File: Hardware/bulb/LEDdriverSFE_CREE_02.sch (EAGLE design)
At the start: 27 parts, among them U1 ZXLD1360, U2 ZXLD1360, U3 ZXLD1360, U4 ZXLD1360, U5 SFW10R-1STE1LF, X1 52745-1090, X2 52745-1090

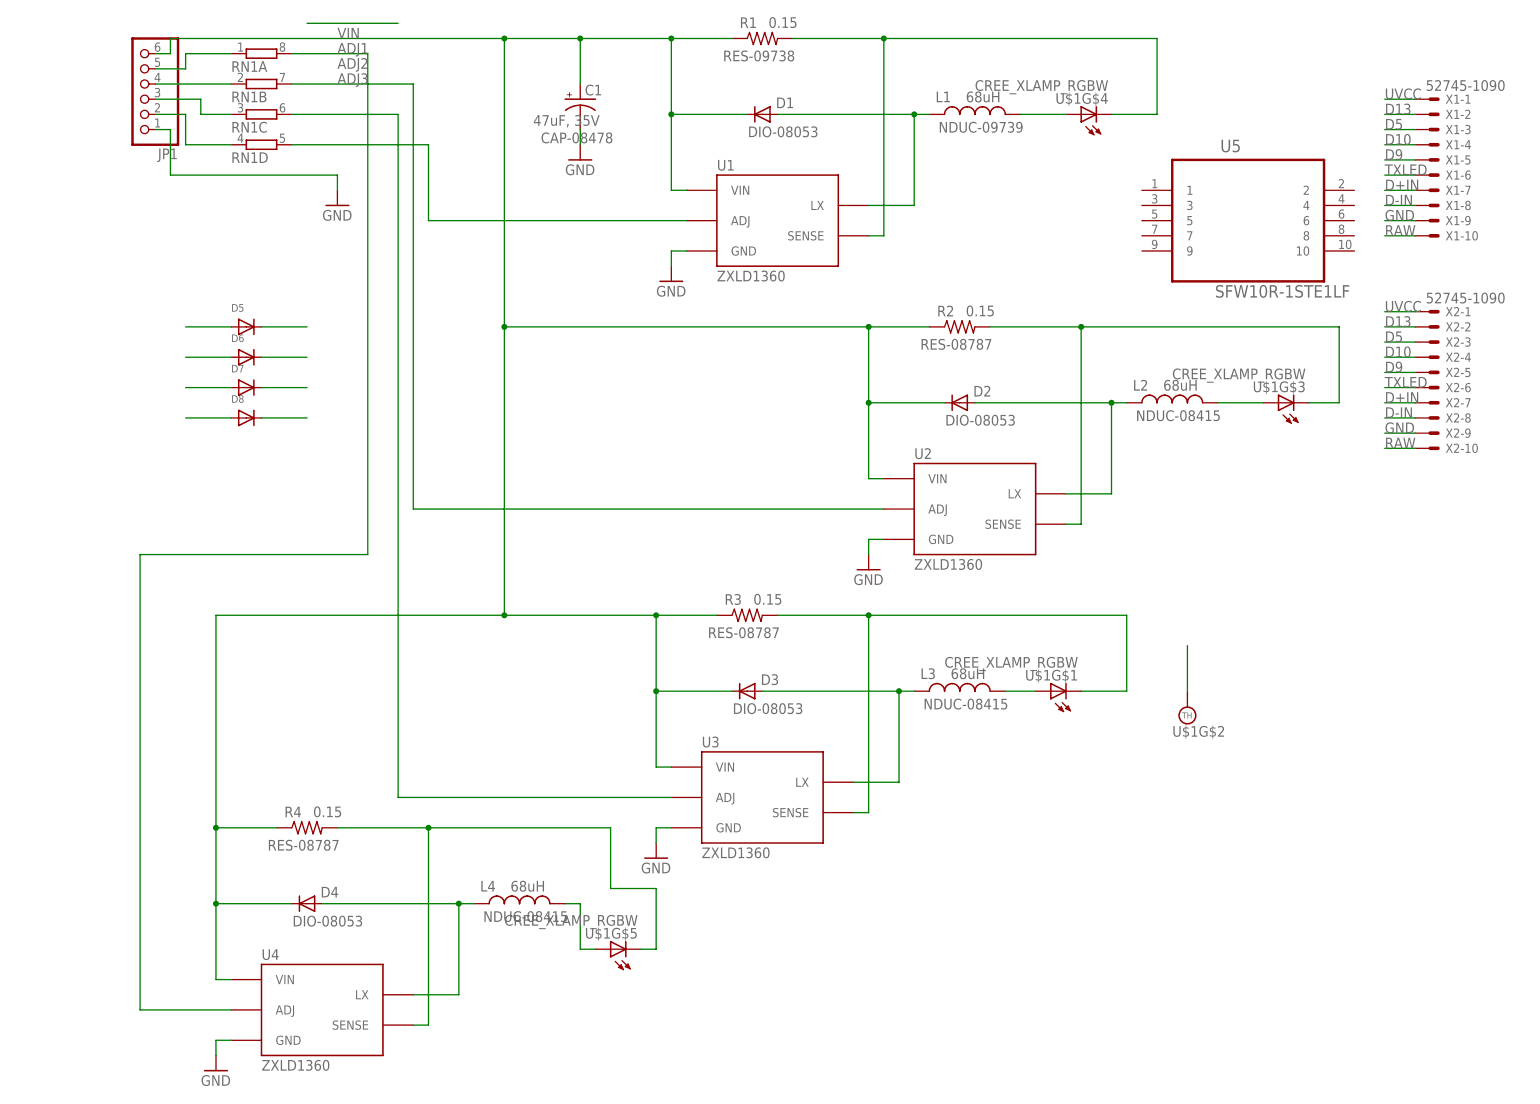
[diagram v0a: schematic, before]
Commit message: updates to api docs and file
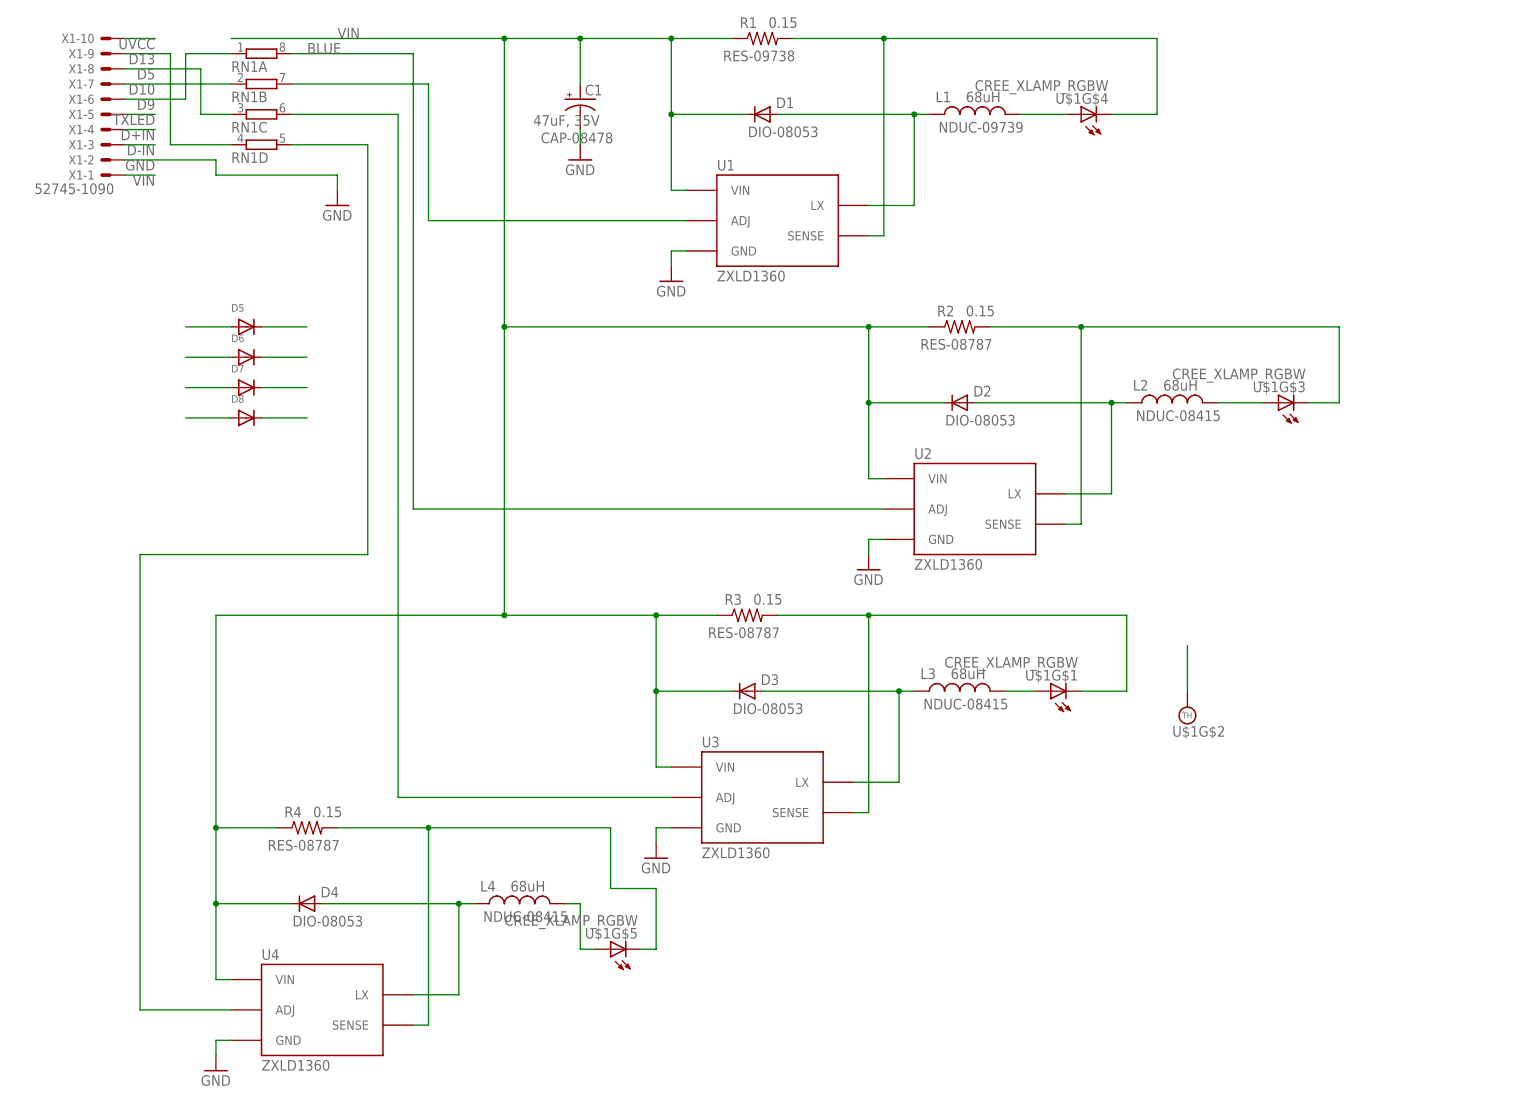
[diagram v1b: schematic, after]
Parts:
- removed JP1: (no value), adafruit:PINHD-1X6
- removed U5: SFW10R-1STE1LF, FCI_By_element14_Batch_1:SFW10R-1STE1LF
- removed X2: 52745-1090, con-molex:52745-1090
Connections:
- net ADJ3 renamed WHITE
- removed net ADJ1: RN1D.2, U1.ADJ
- removed net ADJ2: RN1B.2, U2.ADJ
- removed net BLUEIN: D7.C, JP1.4, RN1B.1
- removed net GREENIN: D6.C, JP1.2, RN1D.1
- removed net N$13: RN1A.2, U4.ADJ
- removed net N$14: D5.A
- removed net N$17: D6.A
- removed net N$20: D7.A
- removed net N$21: D8.A
- removed net RAW: X1-10.S, X2-10.S
- removed net REDIN: D5.C, JP1.5, RN1A.1
- removed net WHITEIN: D8.C, JP1.3, RN1C.1
- new net BLUE: RN1A.2, U2.ADJ
- new net GREEN: RN1B.2, U1.ADJ
- new net RED: RN1D.2, U4.ADJ
- net D+IN: now also X1-4.S; no longer X1-7.S, X2-7.S
- net D-IN: now also X1-3.S; no longer X1-8.S, X2-8.S
- net D10: now also D6.C, RN1B.1, X1-7.S; no longer X1-4.S, X2-4.S
- net D13: now also D7.C, RN1D.1, X1-9.S; no longer X1-2.S, X2-2.S
- net D5: now also D8.C, RN1C.1, X1-8.S; no longer X1-3.S, X2-3.S
- net D9: now also D5.C, RN1A.1, X1-6.S; no longer X1-5.S, X2-5.S
- net GND: now also D5.A, D6.A, D7.A, D8.A, X1-2.S; no longer JP1.1, X1-9.S, X2-9.S
- net TXLED: now also X1-5.S; no longer X1-6.S, X2-6.S
- net UVCC: now also X1-10.S; no longer X1-1.S, X2-1.S
- net VIN: now also X1-1.S; no longer JP1.6
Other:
- moved on the sheet: X1-1, X1-10, X1-2, X1-3, X1-4, X1-5, X1-6, X1-7, X1-8, X1-9
